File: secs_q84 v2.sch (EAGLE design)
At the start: 105 parts, among them IC1 MAX203ECWP, IC2 REF3440TIDBVR, IC3 ADP151AUJZ-3.3-R7, IC4 PIC18F47Q84-I_PT, IC5 MCZ33996EK, IC6 74HC125D, IC7 TIC12400DCPR

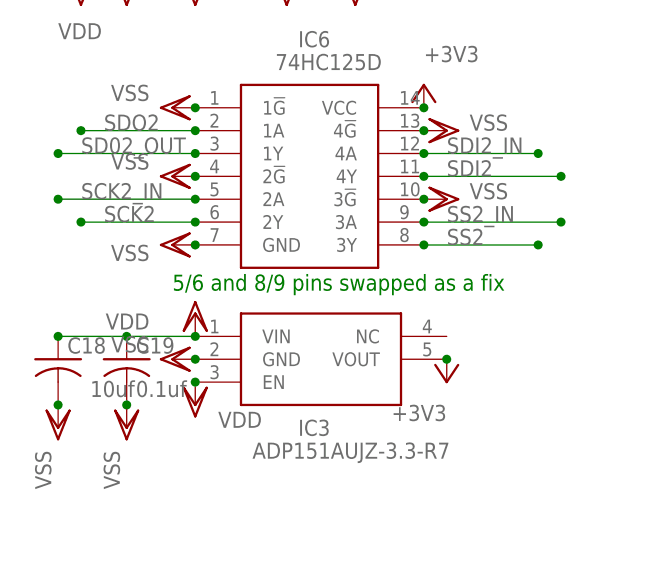
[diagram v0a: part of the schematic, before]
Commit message: add frame
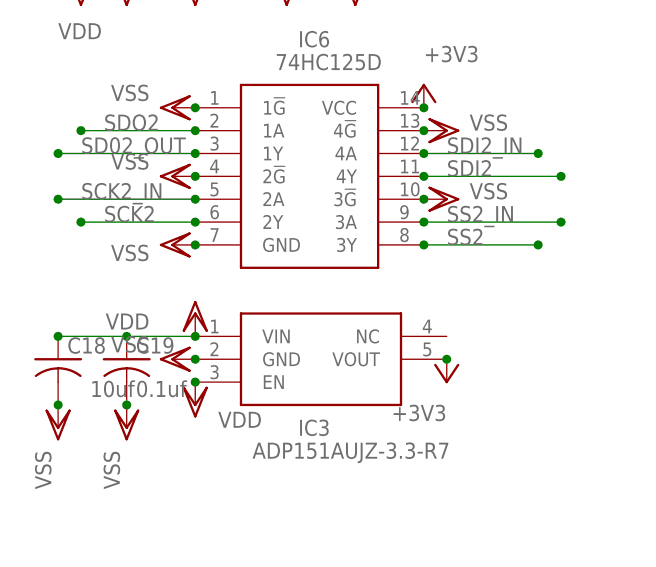
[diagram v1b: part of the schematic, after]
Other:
- note removed: "5/6 and 8/9 pins swapped as a fix"
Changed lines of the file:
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@@
 <part name="VDD27" library="supply1" library_urn="urn:adsk.eagle:library:371" deviceset="VDD" device=""/>
 <part name="P+3" library="supply1" library_urn="urn:adsk.eagle:library:371" deviceset="VCC" device=""/>
+<part name="FRAME1" library="frames" library_urn="urn:adsk.eagle:library:229" deviceset="FRAME_C_L" device=""/>
 </parts>
 <sheets>
 <sheet>
 <plain>
-<text x="332.74" y="-20.32" size="1.778" layer="91">5/6 and 8/9 pins swapped as a fix</text>
 </plain>
 <instances>
@@
 <attribute name="VALUE" x="58.42" y="71.12" size="1.778" layer="96" rot="R180"/>
 </instance>
+<instance part="FRAME1" gate="G$1" x="-142.24" y="-223.52" smashed="yes"/>
+<instance part="FRAME1" gate="G$2" x="309.88" y="-223.52" smashed="yes">
+<attribute name="LAST_DATE_TIME" x="322.58" y="-222.25" size="2.54" layer="94"/>
+<attribute name="SHEET" x="396.24" y="-222.25" size="2.54" layer="94"/>
+<attribute name="DRAWING_NAME" x="327.66" y="-204.47" size="2.54" layer="94"/>
+</instance>
 </instances>

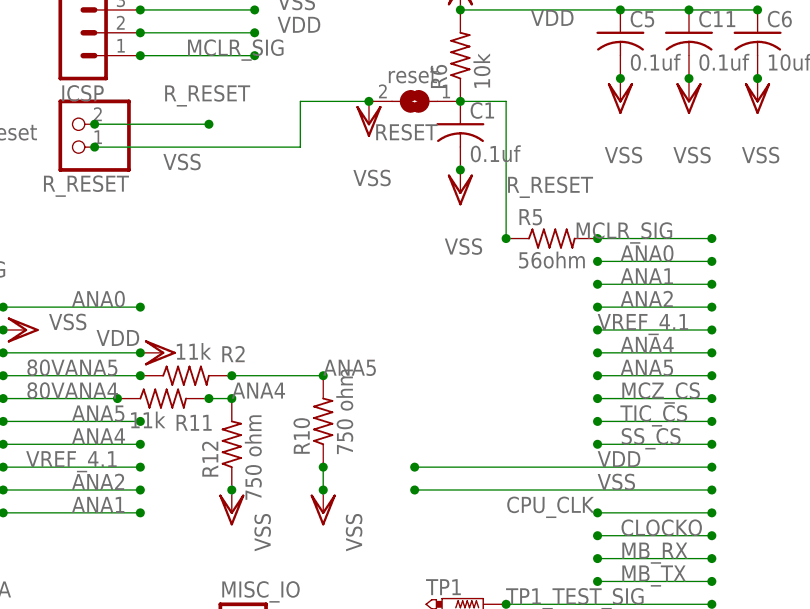
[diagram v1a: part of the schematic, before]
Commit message: PCB updates:wq
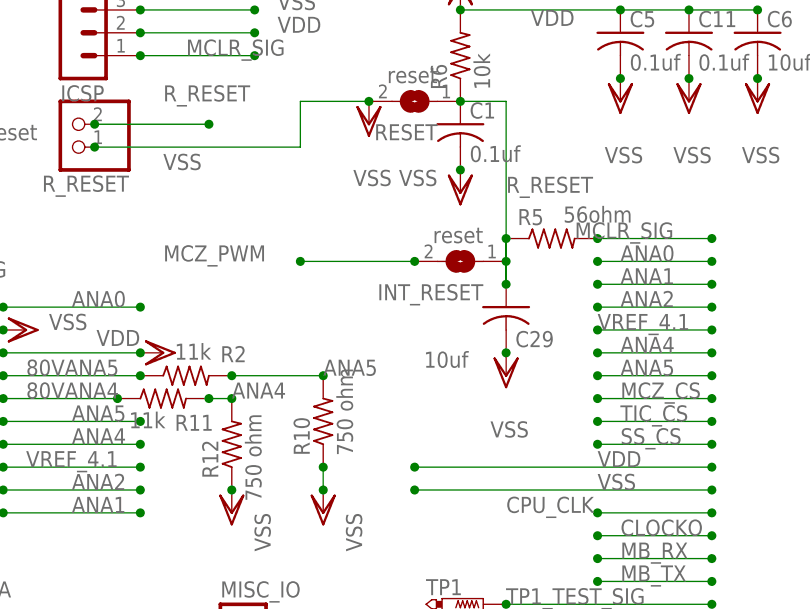
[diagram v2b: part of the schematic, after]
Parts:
- added C29: 10uf, rcl:C-USC0805
- added INT_RESET: reset, jumper:SJ
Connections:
- net MCZ_PWM: now also INT_RESET.2
- net R_RESET: now also C29.1, INT_RESET.1
- net VSS: now also C29.2
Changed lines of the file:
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@@
 <part name="P+3" library="supply1" library_urn="urn:adsk.eagle:library:371" deviceset="VCC" device=""/>
 <part name="FRAME1" library="frames" library_urn="urn:adsk.eagle:library:229" deviceset="FRAME_C_L" device=""/>
+<part name="C29" library="rcl" library_urn="urn:adsk.eagle:library:334" deviceset="C-US" device="C0805" package3d_urn="urn:adsk.eagle:package:23617/2" value="10uf"/>
+<part name="VSS73" library="supply1" library_urn="urn:adsk.eagle:library:371" deviceset="VSS" device=""/>
+<part name="INT_RESET" library="jumper" library_urn="urn:adsk.eagle:library:252" deviceset="SJ" device="" package3d_urn="urn:adsk.eagle:package:15471/1" value="reset"/>
 </parts>
 <sheets>
@@
 <instance part="R5" gate="G$1" x="20.32" y="66.04" smashed="yes">
 <attribute name="NAME" x="16.51" y="67.5386" size="1.778" layer="95"/>
-<attribute name="VALUE" x="16.51" y="62.738" size="1.778" layer="96"/>
+<attribute name="VALUE" x="21.59" y="67.818" size="1.778" layer="96"/>
 </instance>
 <instance part="R6" gate="G$1" x="10.16" y="86.36" smashed="yes" rot="R90">
@@
 </instance>
 <instance part="VSS6" gate="G$1" x="10.16" y="71.12" smashed="yes">
-<attribute name="VALUE" x="12.7" y="66.04" size="1.778" layer="96" rot="R180"/>
+<attribute name="VALUE" x="7.62" y="73.66" size="1.778" layer="96" rot="R180"/>
 </instance>
 <instance part="C2" gate="G$1" x="93.98" y="-5.08" smashed="yes">
@@
 <instance part="FRAME1" gate="G$2" x="309.88" y="-223.52" smashed="yes">
 <attribute name="LAST_DATE_TIME" x="322.58" y="-222.25" size="2.54" layer="94"/>
-<attribute name="SHEET" x="396.24" y="-222.25" size="2.54" layer="94"/>
+<attribute name="SHEET" x="383.54" y="-196.85" size="2.54" layer="94" display="both"/>
 <attribute name="DRAWING_NAME" x="327.66" y="-204.47" size="2.54" layer="94"/>
 </instance>
+<instance part="C29" gate="G$1" x="15.24" y="58.42" smashed="yes">
+<attribute name="NAME" x="16.256" y="53.975" size="1.778" layer="95"/>
+<attribute name="VALUE" x="6.096" y="51.689" size="1.778" layer="96"/>
+</instance>
+<instance part="VSS73" gate="G$1" x="15.24" y="50.8" smashed="yes">
+<attribute name="VALUE" x="17.78" y="45.72" size="1.778" layer="96" rot="R180"/>
+</instance>
+<instance part="INT_RESET" gate="1" x="10.16" y="63.5" smashed="yes" rot="R180">
+<attribute name="NAME" x="12.7" y="60.96" size="1.778" layer="95" rot="R180"/>
+<attribute name="VALUE" x="12.7" y="67.31" size="1.778" layer="96" rot="R180"/>
+</instance>
 </instances>
 <busses>
@@
 <junction x="170.18" y="-172.72"/>
 </segment>
+<segment>
+<pinref part="C29" gate="G$1" pin="2"/>
+<pinref part="VSS73" gate="G$1" pin="VSS"/>
+<junction x="15.24" y="53.34"/>
+</segment>
 </net>
 <net name="CPU_CLK" class="0">
@@
 <segment>
 <pinref part="R5" gate="G$1" pin="1"/>
-<wire x1="15.24" y1="66.04" x2="15.24" y2="81.28" width="0.1524" layer="91"/>
+<wire x1="15.24" y1="60.96" x2="15.24" y2="63.5" width="0.1524" layer="91"/>
 <pinref part="R6" gate="G$1" pin="1"/>
 <pinref part="C1" gate="G$1" pin="1"/>
+<wire x1="15.24" y1="63.5" x2="15.24" y2="66.04" width="0.1524" layer="91"/>
+<wire x1="15.24" y1="66.04" x2="15.24" y2="81.28" width="0.1524" layer="91"/>
 <wire x1="15.24" y1="81.28" x2="10.16" y2="81.28" width="0.1524" layer="91"/>
 <junction x="10.16" y="81.28"/>
-<junction x="15.24" y="66.04"/>
+<junction x="15.24" y="60.96"/>
 <pinref part="RESET" gate="1" pin="1"/>
 <label x="15.24" y="71.12" size="1.778" layer="95"/>
+<pinref part="C29" gate="G$1" pin="1"/>
+<wire x1="15.24" y1="60.96" x2="15.24" y2="63.5" width="0.1524" layer="91"/>
+<junction x="15.24" y="66.04"/>
+<pinref part="INT_RESET" gate="1" pin="1"/>
+<wire x1="15.24" y1="63.5" x2="15.24" y2="66.04" width="0.1524" layer="91"/>
+<junction x="15.24" y="63.5"/>
 </segment>
 <segment>
@@
 <label x="124.46" y="-58.42" size="1.778" layer="95"/>
 </segment>
+<segment>
+<wire x1="-7.62" y1="63.5" x2="5.08" y2="63.5" width="0.1524" layer="91"/>
+<pinref part="INT_RESET" gate="1" pin="2"/>
+<junction x="5.08" y="63.5"/>
+<junction x="-7.62" y="63.5"/>
+<label x="-22.86" y="63.5" size="1.778" layer="95"/>
+</segment>
 </net>
 <net name="SDI2" class="0">
@@
 </sheet>
 </sheets>
+<errors>
+</errors>
 </schematic>
 </drawing>

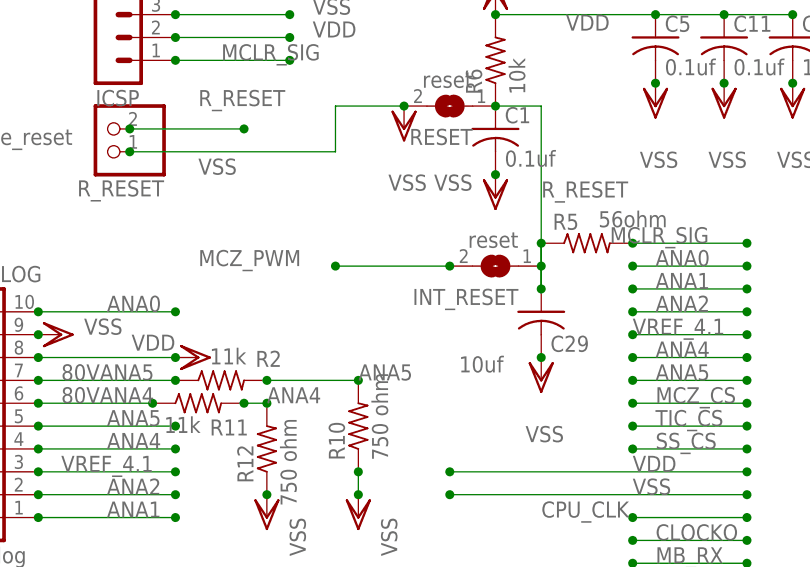
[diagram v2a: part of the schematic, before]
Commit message: up
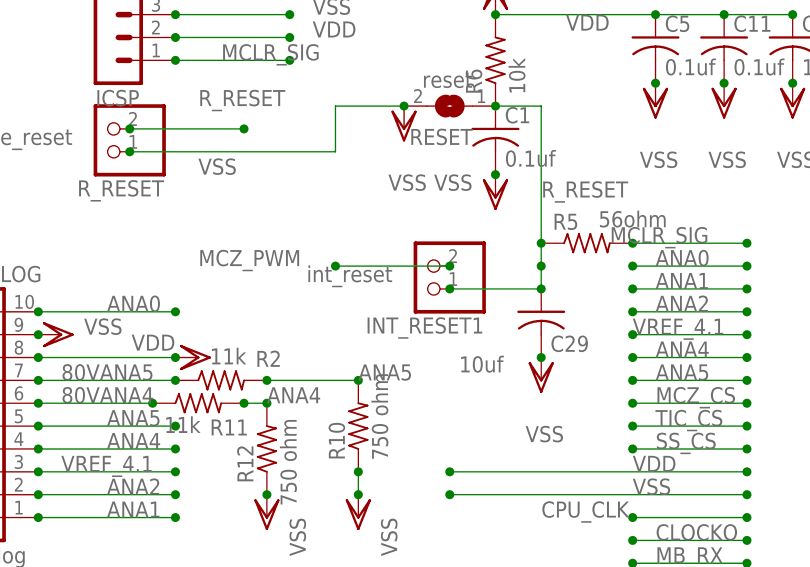
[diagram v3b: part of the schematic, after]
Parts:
- removed INT_RESET: reset, jumper:SJ
- added INT_RESET1: int_reset, pinhead:PINHD-1X2
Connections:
- net MCZ_PWM: now also INT_RESET1.2; no longer INT_RESET.2
- net R_RESET: now also INT_RESET1.1; no longer INT_RESET.1
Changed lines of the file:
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@@
 <part name="C29" library="rcl" library_urn="urn:adsk.eagle:library:334" deviceset="C-US" device="C0805" package3d_urn="urn:adsk.eagle:package:23617/2" value="10uf"/>
 <part name="VSS73" library="supply1" library_urn="urn:adsk.eagle:library:371" deviceset="VSS" device=""/>
-<part name="INT_RESET" library="jumper" library_urn="urn:adsk.eagle:library:252" deviceset="SJ" device="" package3d_urn="urn:adsk.eagle:package:15471/1" value="reset"/>
+<part name="INT_RESET1" library="pinhead" library_urn="urn:adsk.eagle:library:325" deviceset="PINHD-1X2" device="" package3d_urn="urn:adsk.eagle:package:22435/2" value="int_reset"/>
 </parts>
 <sheets>
@@
 <attribute name="VALUE" x="17.78" y="45.72" size="1.778" layer="96" rot="R180"/>
 </instance>
-<instance part="INT_RESET" gate="1" x="10.16" y="63.5" smashed="yes" rot="R180">
-<attribute name="NAME" x="12.7" y="60.96" size="1.778" layer="95" rot="R180"/>
-<attribute name="VALUE" x="12.7" y="67.31" size="1.778" layer="96" rot="R180"/>
+<instance part="INT_RESET1" gate="G$1" x="2.54" y="63.5" smashed="yes" rot="R180">
+<attribute name="NAME" x="8.89" y="57.785" size="1.778" layer="95" rot="R180"/>
+<attribute name="VALUE" x="-1.27" y="63.5" size="1.778" layer="96" rot="R180"/>
 </instance>
 </instances>
@@
 <segment>
 <pinref part="R5" gate="G$1" pin="1"/>
-<wire x1="15.24" y1="60.96" x2="15.24" y2="63.5" width="0.1524" layer="91"/>
 <pinref part="R6" gate="G$1" pin="1"/>
 <pinref part="C1" gate="G$1" pin="1"/>
-<wire x1="15.24" y1="63.5" x2="15.24" y2="66.04" width="0.1524" layer="91"/>
 <wire x1="15.24" y1="66.04" x2="15.24" y2="81.28" width="0.1524" layer="91"/>
 <wire x1="15.24" y1="81.28" x2="10.16" y2="81.28" width="0.1524" layer="91"/>
@@
 <wire x1="15.24" y1="60.96" x2="15.24" y2="63.5" width="0.1524" layer="91"/>
 <junction x="15.24" y="66.04"/>
-<pinref part="INT_RESET" gate="1" pin="1"/>
 <wire x1="15.24" y1="63.5" x2="15.24" y2="66.04" width="0.1524" layer="91"/>
 <junction x="15.24" y="63.5"/>
+<pinref part="INT_RESET1" gate="G$1" pin="1"/>
+<wire x1="5.08" y1="60.96" x2="15.24" y2="60.96" width="0.1524" layer="91"/>
+<junction x="5.08" y="60.96"/>
 </segment>
 <segment>
@@
 <segment>
 <wire x1="-7.62" y1="63.5" x2="5.08" y2="63.5" width="0.1524" layer="91"/>
-<pinref part="INT_RESET" gate="1" pin="2"/>
-<junction x="5.08" y="63.5"/>
 <junction x="-7.62" y="63.5"/>
 <label x="-22.86" y="63.5" size="1.778" layer="95"/>
-</segment>
-</net>
+<pinref part="INT_RESET1" gate="G$1" pin="2"/>
+<junction x="5.08" y="63.5"/>
+</segment>
+</net>
